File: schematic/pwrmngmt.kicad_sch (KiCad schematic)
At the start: 46 parts, among them U10 BSD316, U11 BSD316, U12 PC817, U13 PC817, U14 PC817, U15 AS431, U16 LM324, U17 XL6009, U18 PAM2305CGFADJ, U9 BSD316

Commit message: a
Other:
- title: (none) -> Power Managment
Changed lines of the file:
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@@
 (kicad_sch (version 20211123) (generator eeschema)
   (paper "A4")
+  (title_block
+    (title "Power Managment")
+    (date "2022-03-18")
+    (comment 1 "Engineer/Draftsman: Joesphan Lu")
+  )
   (junction (at 251.46 24.13) (diameter 0) (color 0 0 0 0)
   )

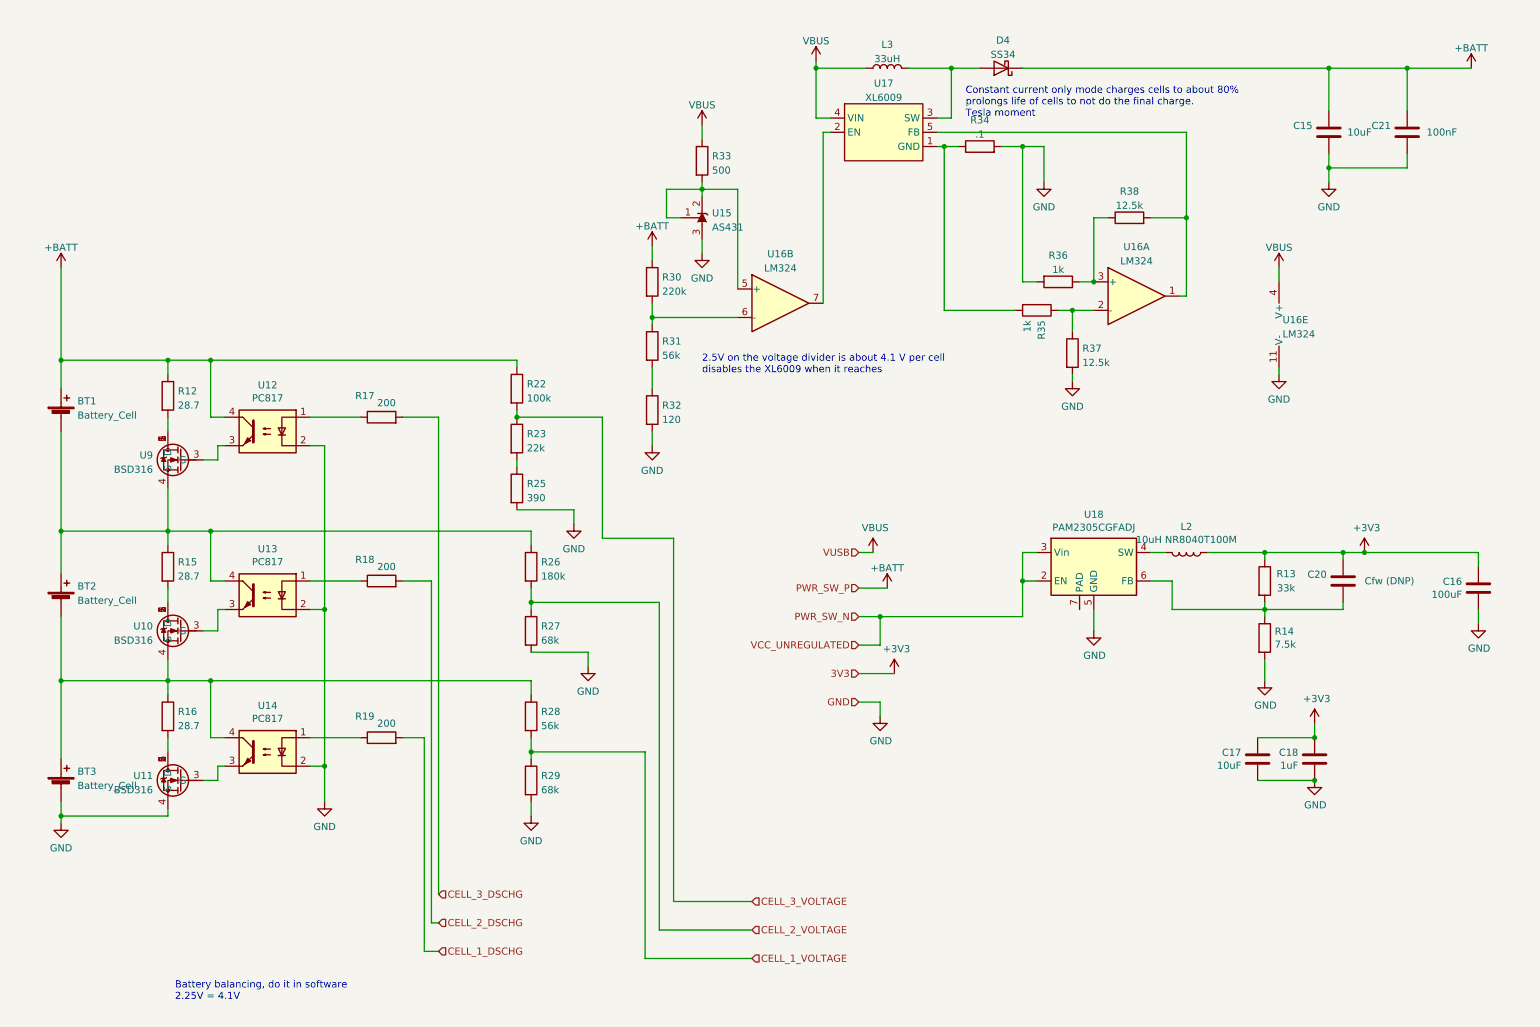
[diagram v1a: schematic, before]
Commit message: e
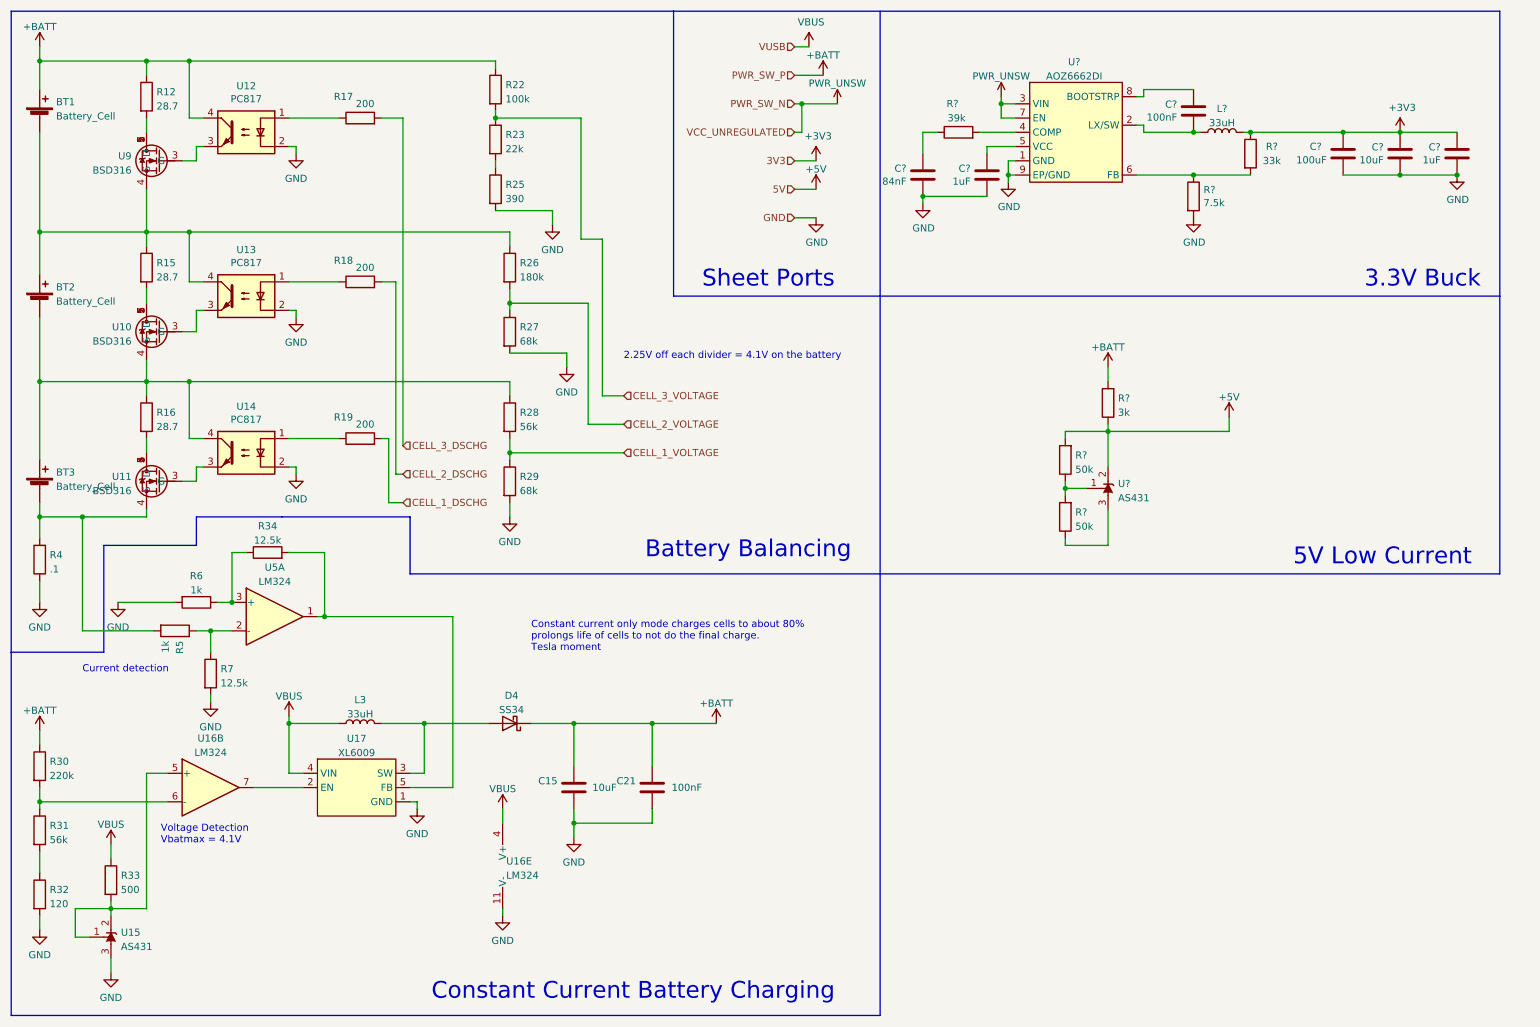
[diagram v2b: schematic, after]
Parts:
- removed C16: 100uF, Capacitor_SMD:C_1210_3225Metric_Pad1.33x2.70mm_HandSolder, symbol Device:C
- removed C17: 10uF, Capacitor_SMD:C_0805_2012Metric_Pad1.18x1.45mm_HandSolder, symbol Device:C
- removed C18: 1uF, Capacitor_SMD:C_0805_2012Metric_Pad1.18x1.45mm_HandSolder, symbol Device:C
- removed C20: Cfw (DNP), Capacitor_SMD:C_0805_2012Metric_Pad1.18x1.45mm_HandSolder, symbol Device:C
- removed L2: 10uH NR8040T100M, Inductor_SMD:L_Taiyo-Yuden_NR-80xx_HandSoldering, symbol Device:L
- removed R13: 33k, Resistor_SMD:R_0805_2012Metric_Pad1.20x1.40mm_HandSolder, symbol Device:R
- removed R14: 7.5k, Resistor_SMD:R_0805_2012Metric_Pad1.20x1.40mm_HandSolder, symbol Device:R
- removed R35, R36: 1k, Resistor_SMD:R_0805_2012Metric_Pad1.20x1.40mm_HandSolder, symbol Device:R
- removed R37, R38: 12.5k, Resistor_SMD:R_0805_2012Metric_Pad1.20x1.40mm_HandSolder, symbol Device:R
- removed unit 1 of U16
- removed U18: PAM2305CGFADJ, Package_DFN_QFN:DFN-6-1EP_2x2mm_P0.65mm_EP1x1.6mm, symbol Regulator_Switching:PAM2305CGFADJ
- added C?: 100nF, Capacitor_SMD:C_0805_2012Metric_Pad1.18x1.45mm_HandSolder, symbol Device:C
- added C?: 84nF, Capacitor_SMD:C_0805_2012Metric_Pad1.18x1.45mm_HandSolder, symbol Device:C
- added C? (x2): 1uF, Capacitor_SMD:C_0805_2012Metric_Pad1.18x1.45mm_HandSolder, symbol Device:C
- added C?: 10uF, Capacitor_SMD:C_0805_2012Metric_Pad1.18x1.45mm_HandSolder, symbol Device:C
- added C?: 100uF, Capacitor_SMD:C_1210_3225Metric_Pad1.33x2.70mm_HandSolder, symbol Device:C
- added L?: 33uH, Inductor_SMD:L_10.4x10.4_H4.8, symbol Device:L
- added R4: .1, Resistor_SMD:R_1206_3216Metric_Pad1.30x1.75mm_HandSolder, symbol Device:R
- added R5, R6: 1k, Resistor_SMD:R_0805_2012Metric_Pad1.20x1.40mm_HandSolder, symbol Device:R
- added R7: 12.5k, Resistor_SMD:R_0805_2012Metric_Pad1.20x1.40mm_HandSolder, symbol Device:R
- added R? (x2): 50k, Resistor_SMD:R_0805_2012Metric_Pad1.20x1.40mm_HandSolder, symbol Device:R
- added R?: 3k, Resistor_SMD:R_0805_2012Metric_Pad1.20x1.40mm_HandSolder, symbol Device:R
- added R?: 39k, Resistor_SMD:R_0805_2012Metric_Pad1.20x1.40mm_HandSolder, symbol Device:R
- added R?: 7.5k, Resistor_SMD:R_0805_2012Metric_Pad1.20x1.40mm_HandSolder, symbol Device:R
- added R?: 33k, Resistor_SMD:R_0805_2012Metric_Pad1.20x1.40mm_HandSolder, symbol Device:R
- added U5: LM324, Package_SO:SOIC-14_3.9x8.7mm_P1.27mm, symbol Amplifier_Operational:LM324
- added U?: AOZ6662DI, 1KicadLib:DFN_8_3x3mm_EP_1.25x2.7mm, symbol 1KicadLib:AOZ6662DI
- added U?: AS431, Package_TO_SOT_SMD:SOT-23_Handsoldering, symbol 1KicadLib:AS431
- D4: footprint Diode_SMD:D_SMC_Handsoldering -> Diode_SMD:D_SMA_Handsoldering
- L3: footprint Inductor_SMD:L_12x12mm_H4.5mm -> Inductor_SMD:L_10.4x10.4_H4.8
- R34: value .1 -> 12.5k; footprint Resistor_SMD:R_1206_3216Metric_Pad1.30x1.75mm_HandSolder -> Resistor_SMD:R_0805_2012Metric_Pad1.20x1.40mm_HandSolder
- U12, U13, U14: footprint Package_SO:SOP-4_3.8x4.1mm_P2.54mm -> Package_DIP:DIP-4_W7.62mm
- U15: footprint Package_TO_SOT_SMD:SOT-23-5_HandSoldering -> Package_TO_SOT_SMD:SOT-23_Handsoldering
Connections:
- net +3V3: now also C?.1, C?.1, C?.1, L?.2, R?.1
- net +BATT: now also R?.2
- net GND: now also U17.1 (GND), C?.2, C?.2, C?.2, C?.2, C?.2, R4.1, R6.2, R7.2, R?.2, U?.1 (GND), U?.9 (EP/GND); no longer BT3.2 (-), R34.2, U11.4 (S)
- net at R34.1: now also R6.1, U5.3 (+); no longer U17.1 (GND)
- net at U17.5 (FB): now also R34.2, U5.1
- new net: BT3.2 (-), R4.2, R5.2, U11.4 (S)
- new net: C?.1, U?.8 (BOOTSTRP)
- new net: C?.2, L?.1, U?.2 (LX/SW)
- new net: R?.1, R?.2, U?.1
- new net: R?.2, U?.4 (COMP)
- new net: C?.1, U?.5 (VCC)
- new net: R?.1, R?.2, U?.6 (FB)
- new net: C?.1, R?.1
- new net: R5.1, R7.1, U5.2 (-)
- new net: R?.1, U?.3
- new net +5V: R?.1, R?.2, U?.2
- new net PWR_UNSW: U?.3 (VIN), U?.7 (EN)
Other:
- note added: "2.25V off each divider = 4.1V on the battery"
- note added: "3.3V Buck"
- note added: "5V Low Current"
- note added: "Battery Balancing"
- note added: "Constant Current Battery Charging"
- note added: "Current detection"
- note added: "Sheet Ports"
- note added: "Voltage Detection Vbatmax = 4.1V"
- note removed: "2.5V on the voltage divider is about 4.1 V per cell disables the XL6009 when it reaches"
- note removed: "Battery balancing, do it in software 2.25V = 4.1V"
- moved on the sheet: BT1, BT2, BT3, C15, C21, D4, L3, R12, R15, R16, R17, R18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
